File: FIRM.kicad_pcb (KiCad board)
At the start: 8 copper layers, 21.3 x 27 mm, 93 parts, among them J1 DM3CS-SF, J2 Conn_01x02_Pin, Q1 IRLML6402, U1 W25Q128JVP, U2 STM32F405RGTx, U3 ADXL371, U5 INA219AxDCN, U6 MIC5219-3.3YM5, U9 A-USBC-20F0-EA-GSR05, X1 32.768khz, Y1 12 MHz

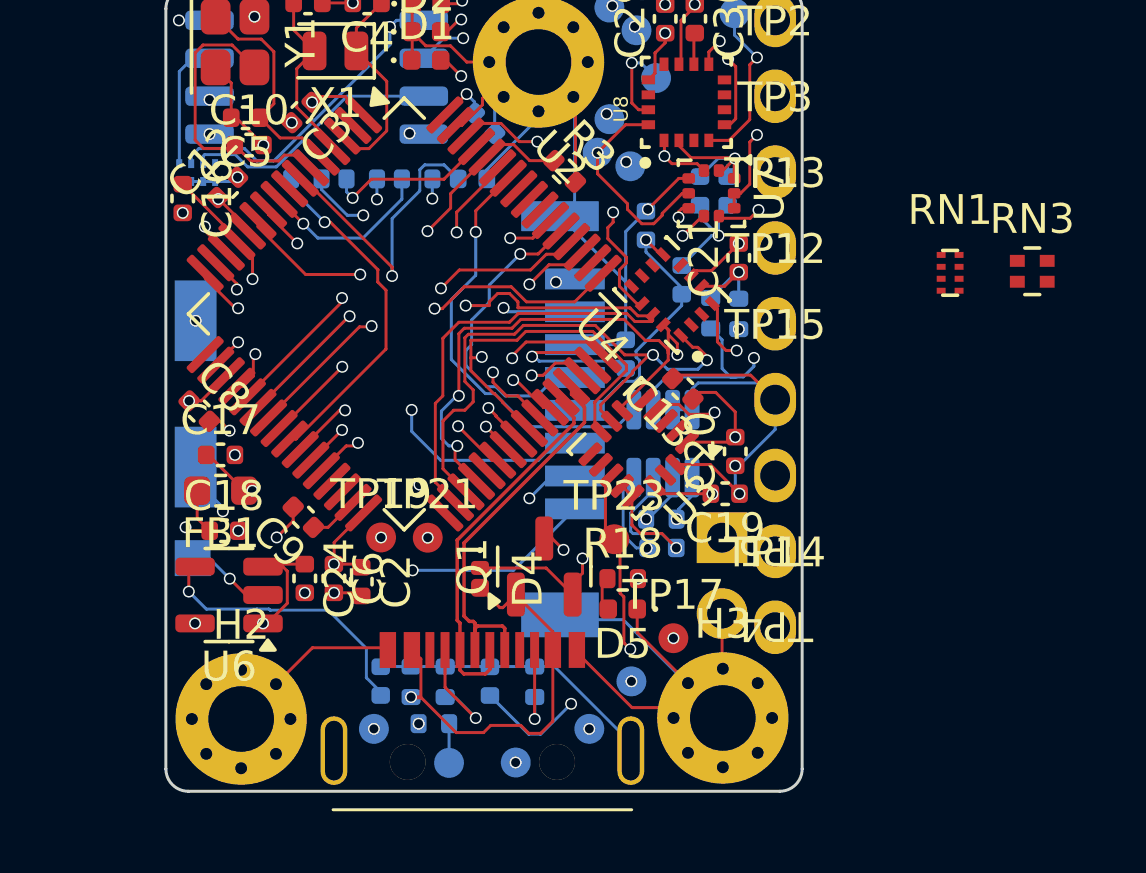
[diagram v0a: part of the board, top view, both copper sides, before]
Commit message: added back resistors
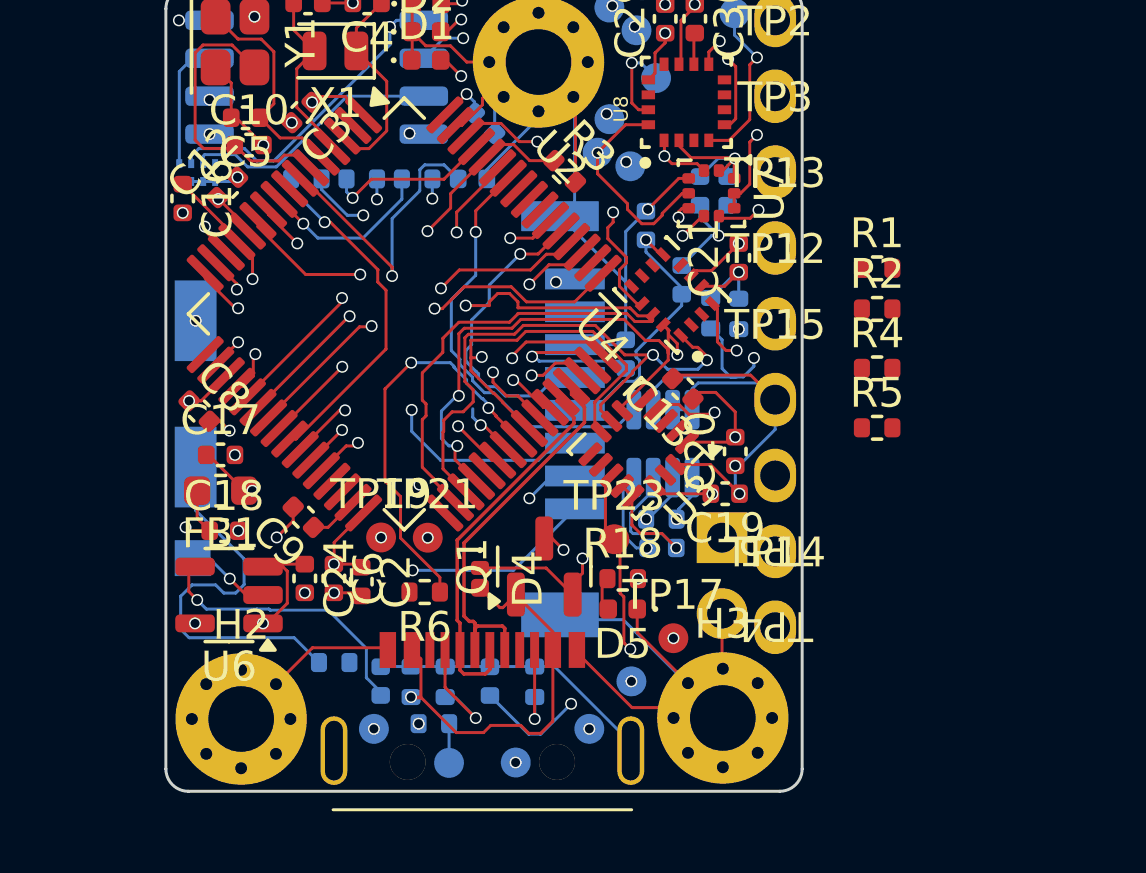
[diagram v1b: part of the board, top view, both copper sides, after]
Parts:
- removed RN1: 47k, connectors:R_Array_YC104
- removed RN3: 47k, connectors:R_Array_EXB-24V
- added R1: 47k, Resistor_SMD:R_0402_1005Metric, F.Cu at (177.2, 84.0)
- added R2: 47k, Resistor_SMD:R_0402_1005Metric, F.Cu at (177.2, 85.4)
- added R4: 47k, Resistor_SMD:R_0402_1005Metric, F.Cu at (177.2, 87.4)
- added R5: 47k, Resistor_SMD:R_0402_1005Metric, F.Cu at (177.2, 89.4)
- added R6: 47k, Resistor_SMD:R_0402_1005Metric, F.Cu at (162.0, 94.9)
- added R7: 47k, Resistor_SMD:R_0402_1005Metric, B.Cu at (159.0, 97.2)
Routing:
- net /SDIO_D1: track 7.58 -> 19.8 mm, vias 2 -> 3
- net /SD_DETECT: track 9.67 -> 21.6 mm, vias 2 -> 1
- net /SDIO_D0: track 8.51 -> 6.93 mm, vias 2 -> 1

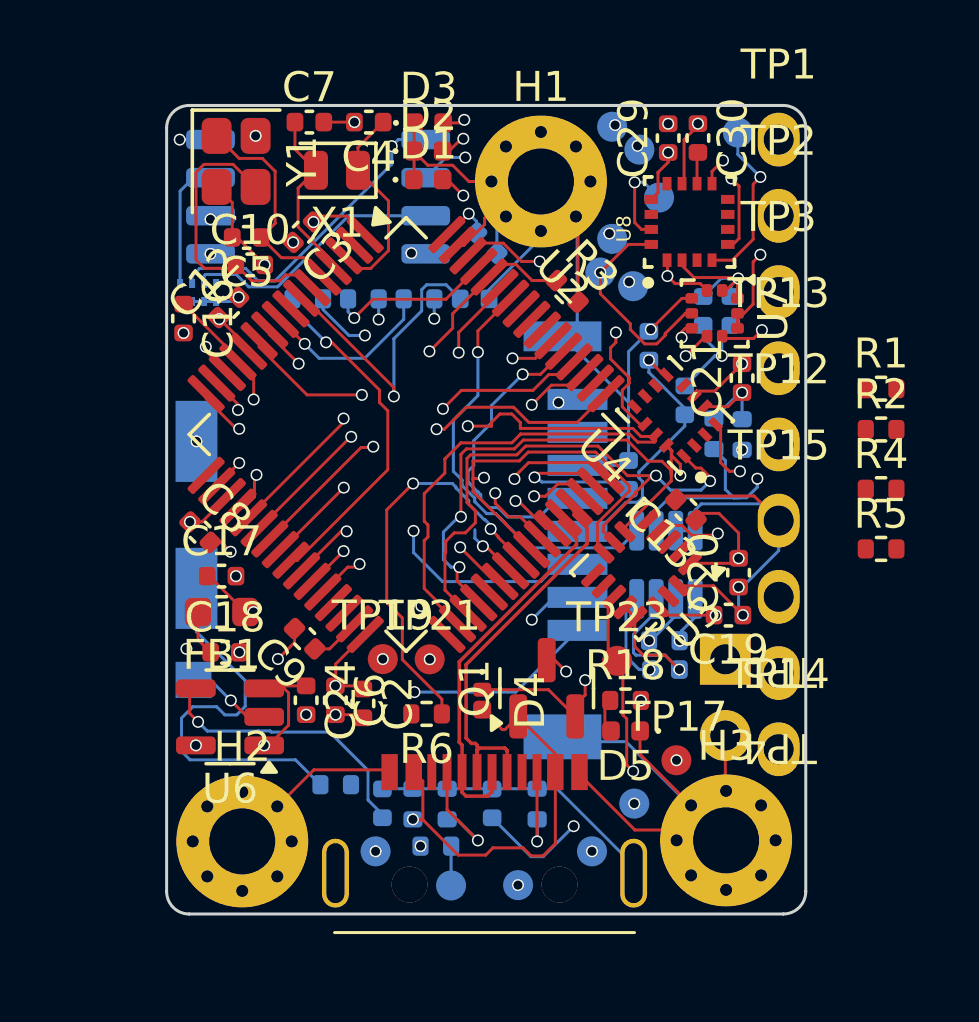
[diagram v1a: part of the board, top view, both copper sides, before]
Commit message: finished routing resistors
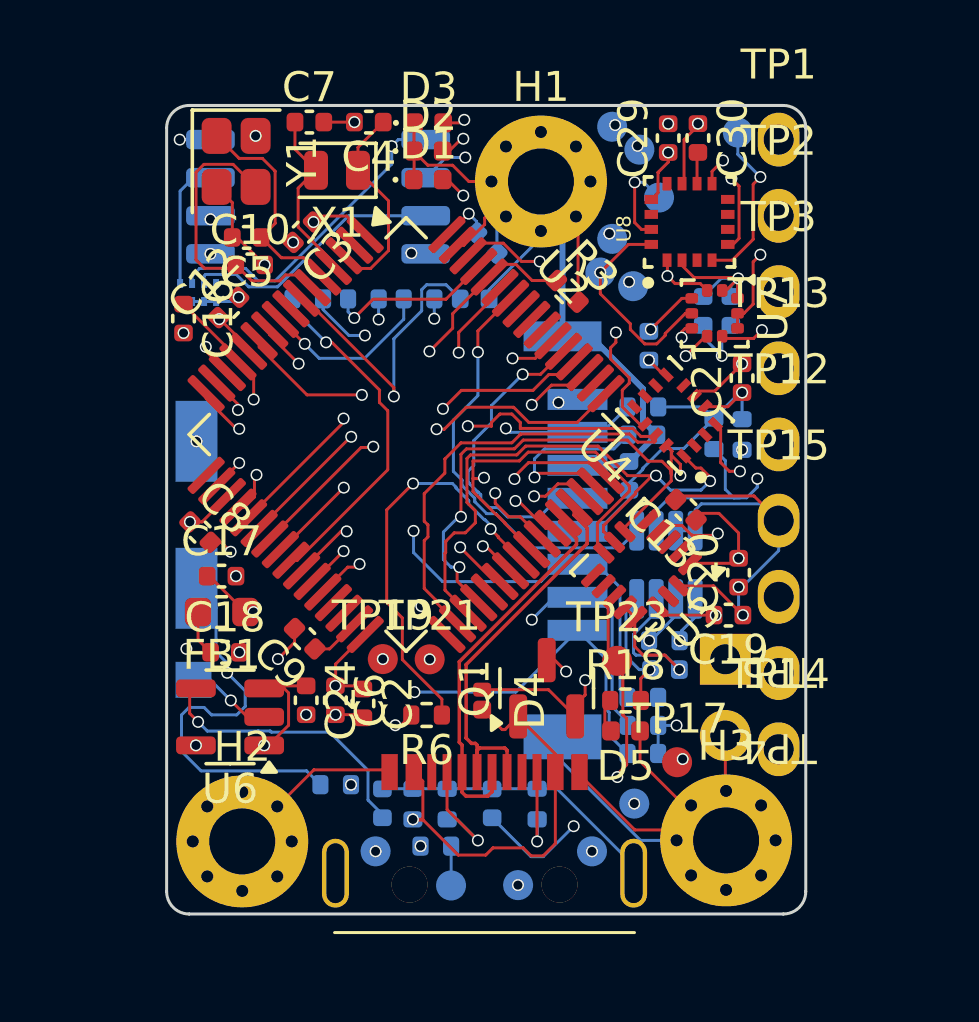
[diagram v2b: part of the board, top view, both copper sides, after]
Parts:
- R1, R2, R4, R5: moved to B.Cu
- moved R1 14.5 mm to (169.2, 96.2)
- moved R2 12.7 mm to (169.2, 95.2)
- moved R4 10.5 mm to (169.2, 94.3)
- moved R5 9.24 mm to (169.2, 84.6)
- moved C11 3.13 mm to (168.7, 86.9)
- moved C14 1.42 mm to (169.2, 85.6), turned to 0 degrees
- moved TP17 0.07 mm to (170.3, 96.5)
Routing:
- net /SDIO_CMD: track 16.4 -> 21.9 mm
- net /SDIO_D3: track 15.2 -> 20.6 mm
- net +3.3V: track 55.8 -> 61.0 mm, vias 18 -> 20
- net /SDIO_D2: track 19.8 -> 24.6 mm
- net /SDIO_D0: track 6.93 -> 10.7 mm, vias 1 -> 2
- net /VCAP2: track 5.00 -> 5.78 mm
- net /SD_DETECT: track 21.6 -> 22.1 mm, vias 1 -> 2

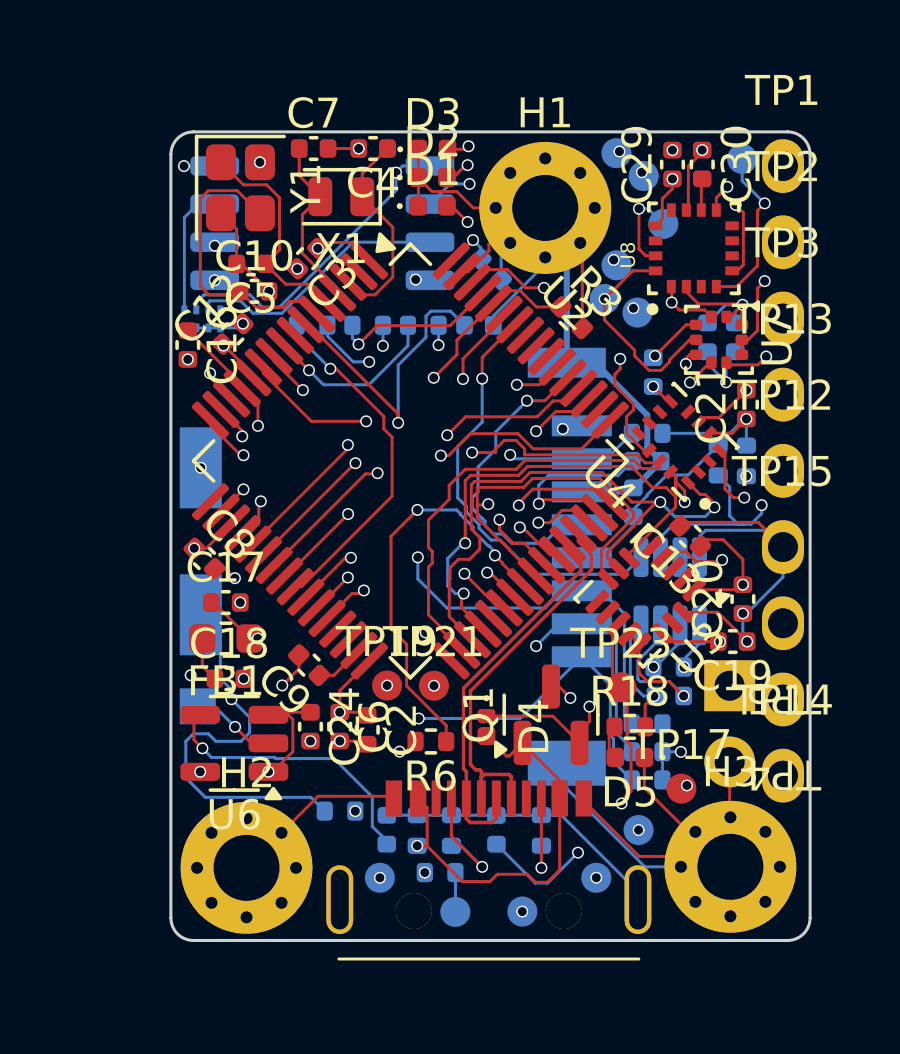
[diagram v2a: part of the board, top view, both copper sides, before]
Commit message: a lil bit of this a lil bit of that
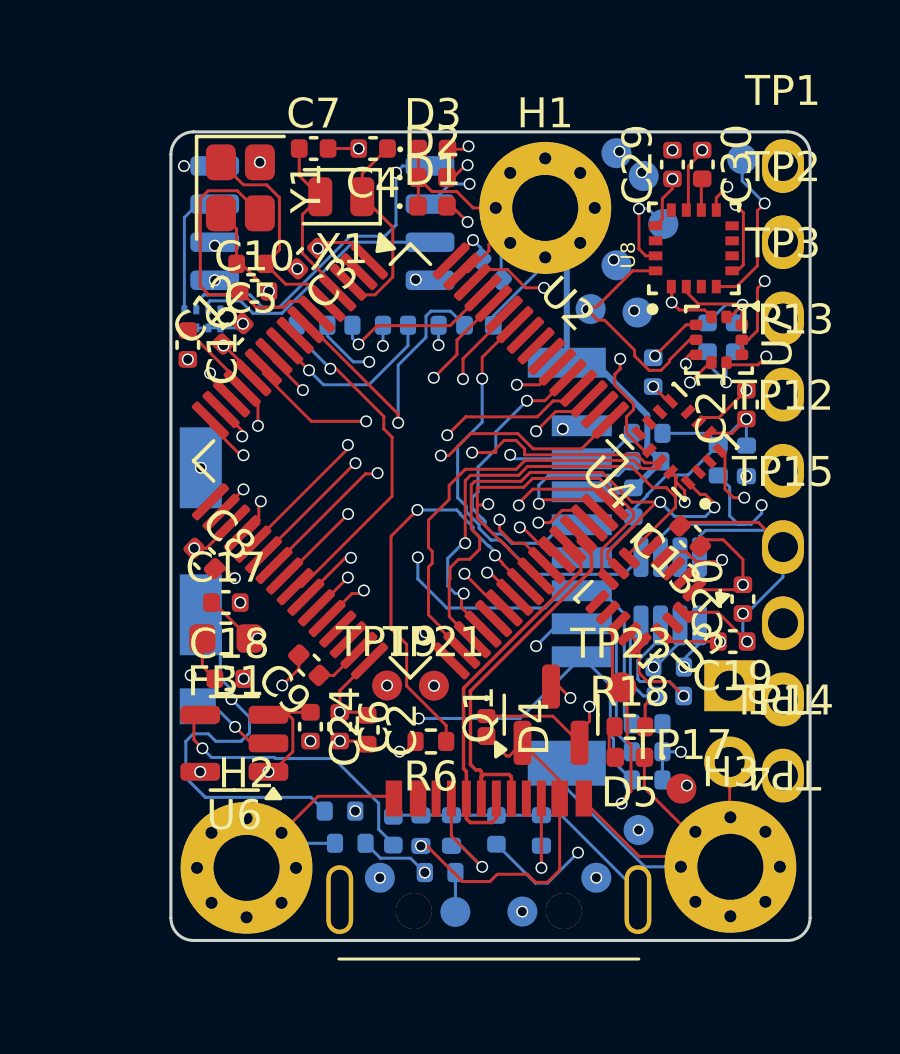
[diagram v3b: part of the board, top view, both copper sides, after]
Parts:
- R3: moved to B.Cu
- moved R3 19.0 mm to (159.3, 98.3), turned to 180 degrees
- moved TP7 0.57 mm to (167.3, 80.5)
- moved C26 0.22 mm to (160.7, 97.9)
- moved R16 0.12 mm to (161.7, 97.9)
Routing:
- net VBUS: track 14.1 -> 11.9 mm
- net /MOSI2: track 36.3 -> 37.7 mm
- net /FLASH_CS: track 26.0 -> 26.7 mm
- net GND: track 109.6 -> 110.1 mm

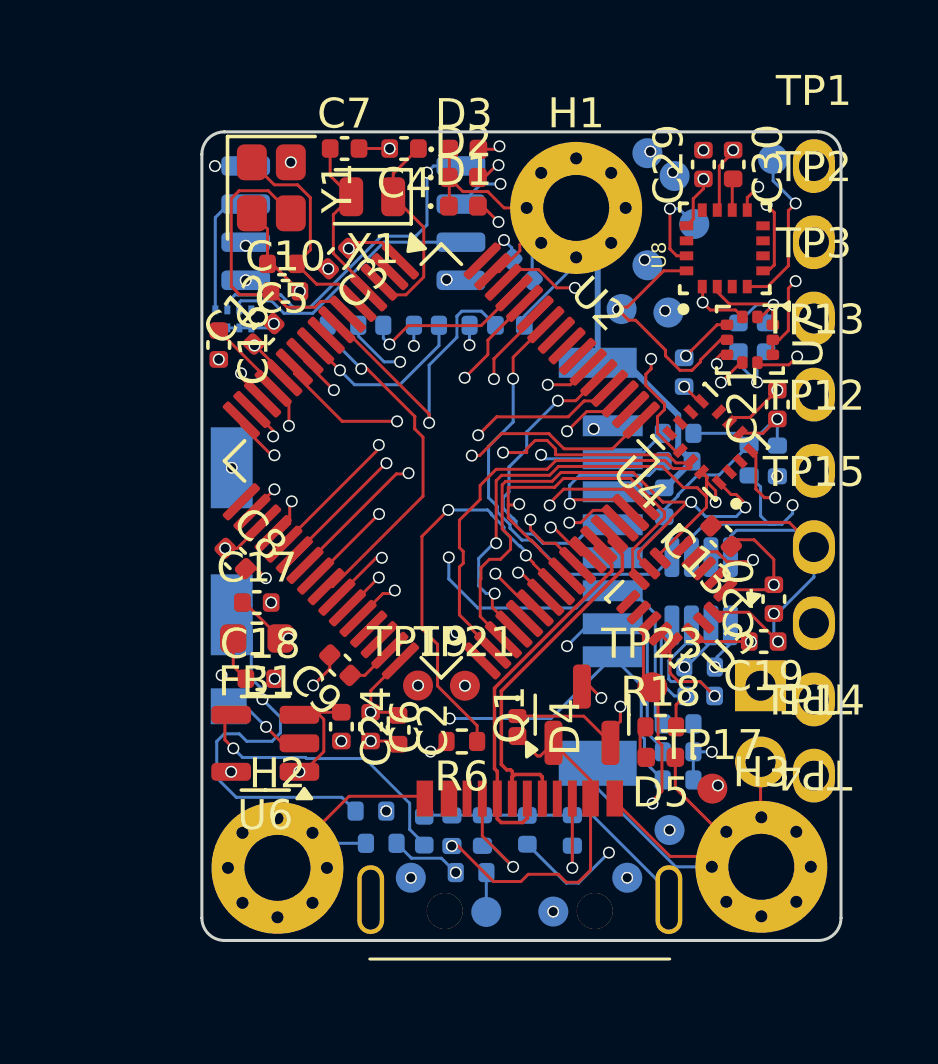
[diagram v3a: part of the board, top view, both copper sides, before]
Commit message: changes
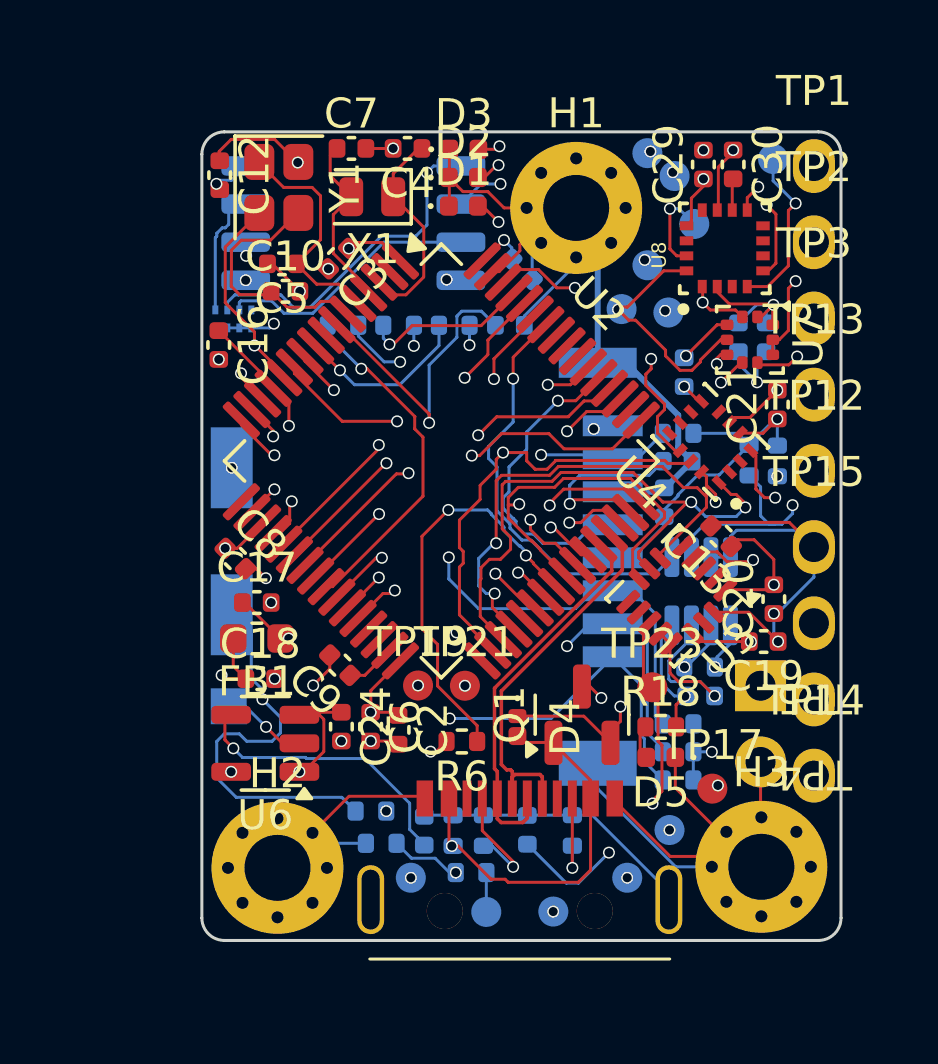
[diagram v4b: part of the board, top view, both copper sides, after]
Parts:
- moved C12 5.49 mm to (153.9, 76.0), turned to -90 degrees
- moved Y1 0.25 mm to (155.9, 76.4)
- moved C7 0.23 mm to (158.3, 75.1)
- moved C4 0.12 mm to (160.2, 75.1)
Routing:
- net GND: track 110.1 -> 117.4 mm
- net /SCK2: track 51.2 -> 44.8 mm
- net /PA9: track 15.1 -> 16.4 mm
- net /HSE_OUT: track 9.08 -> 7.71 mm
- net VBUS: track 11.9 -> 13.0 mm
